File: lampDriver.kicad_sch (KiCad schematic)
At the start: 49 parts, among them IC8 FAN3100TSX, T4 NMOS_GDS-KS_SMD, U1 OPA2356AIDGKR, U3 LM2903, U4 AZ431LANTR

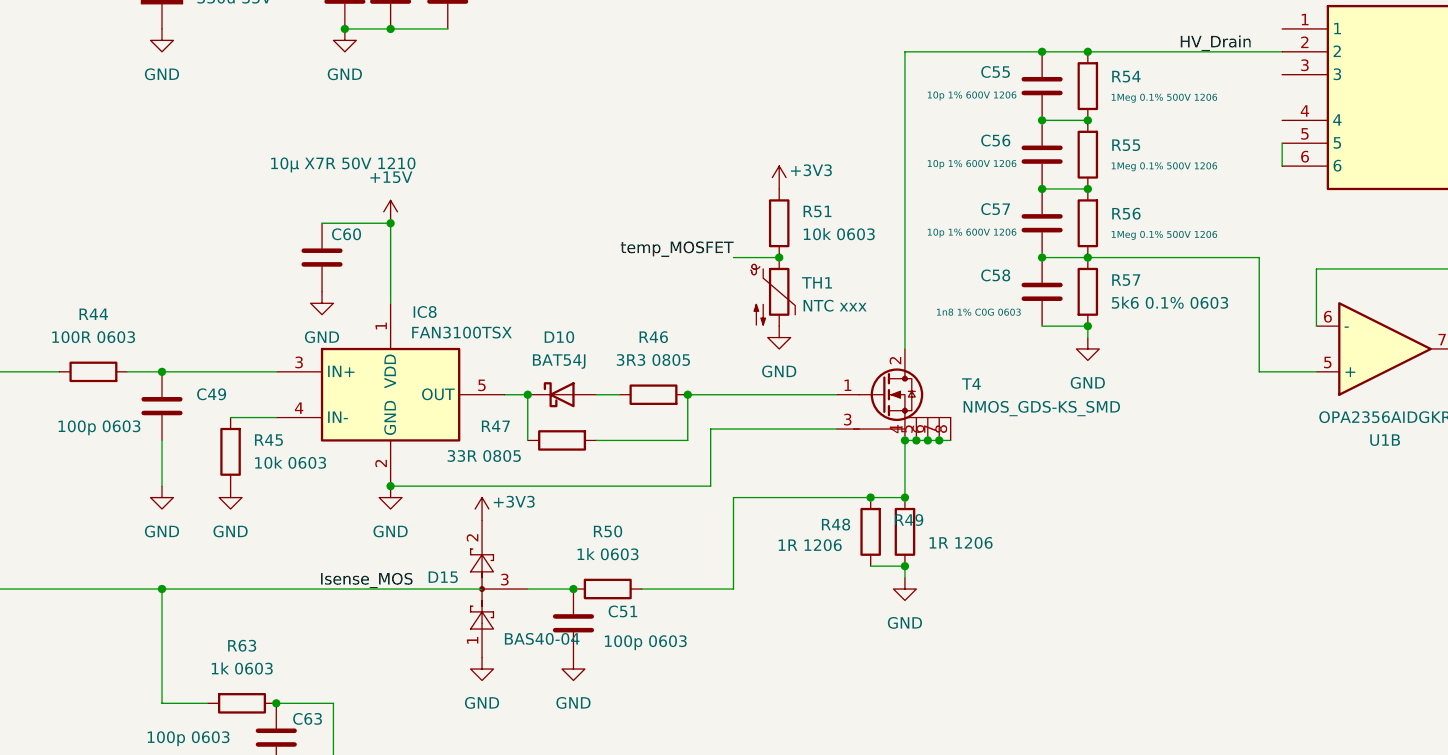
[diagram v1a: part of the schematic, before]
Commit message: 250415_endOfDay
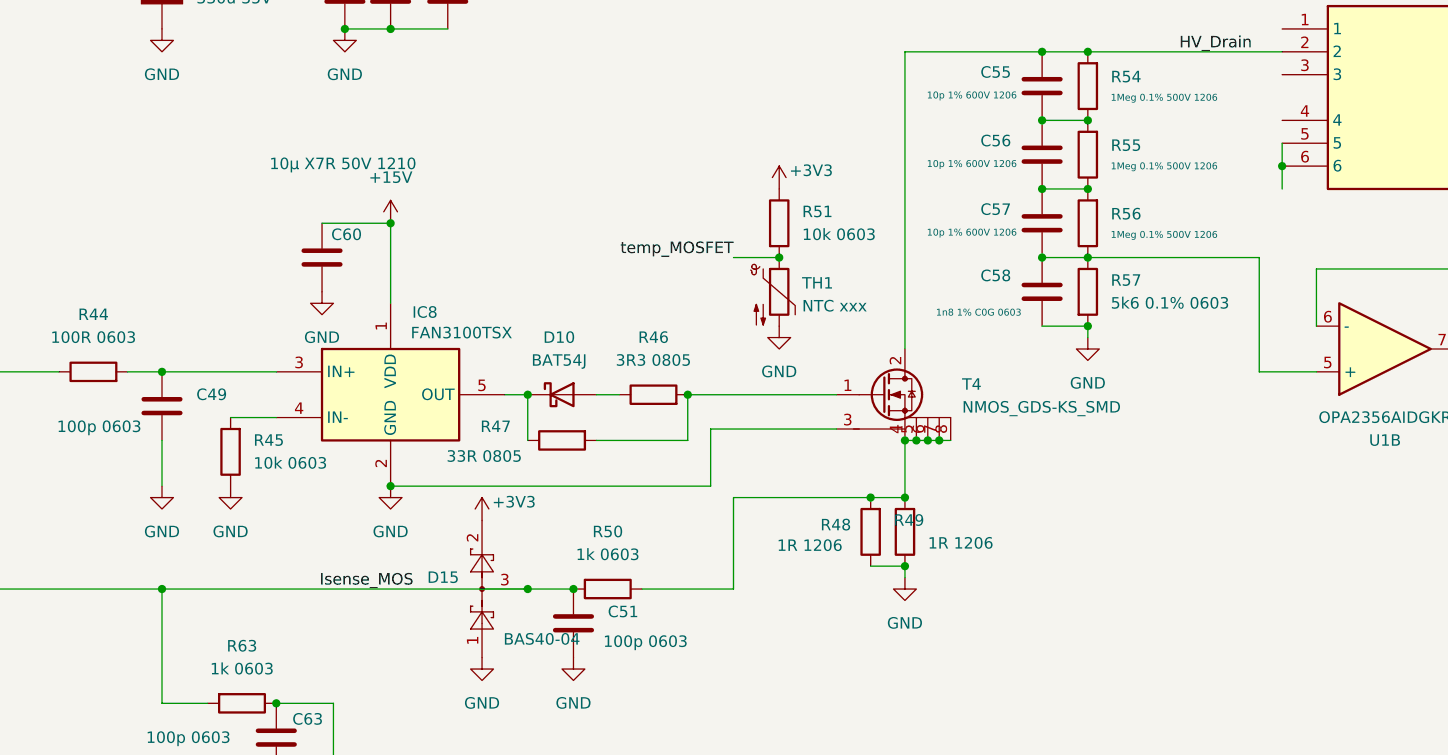
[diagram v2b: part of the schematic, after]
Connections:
- net Isense_MOS: now also C51.1, D15.3, R50.2
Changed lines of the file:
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@@
+	)
+	(junction
+		(at 175.26 60.96)
+		(diameter 0)
+		(color 0 0 0 0)
 	)
 	(junction
@@
 	)
 	(junction
+		(at 91.44 107.95)
+		(diameter 0)
+		(color 0 0 0 0)
+	)
+	(junction
 		(at 76.2 67.31)
 		(diameter 0)
@@
 	(wire
 		(pts
+			(xy 175.26 60.96) (xy 175.26 63.5)
+		)
+		(stroke
+			(width 0)
+			(type default)
+		)
+	)
+	(wire
+		(pts
 			(xy 208.28 50.8) (xy 208.28 71.12)
 		)
@@
 	(wire
 		(pts
-			(xy 50.8 107.95) (xy 86.36 107.95)
+			(xy 50.8 107.95) (xy 91.44 107.95)
 		)
 		(stroke
@@
 			(fill
 				(type none)
+			)
+		)
+	)
+	(netclass_flag ""
+		(length 2.54)
+		(shape round)
+		(at 153.67 63.5 270)
+		(effects
+			(font
+				(size 1.27 1.27)
+			)
+			(justify right bottom)
+		)
+		(property "Net Class" "HV_Drain_div2"
+			(at 157.734 63.246 0)
+			(effects
+				(font
+					(size 1.27 1.27)
+				)
+				(justify left)
+			)
+		)
+		(property "Component Class" ""
+			(at -49.53 8.89 0)
+			(effects
+				(font
+					(size 1.27 1.27)
+					(italic yes)
+				)
+			)
+		)
+	)
+	(netclass_flag ""
+		(length 2.54)
+		(shape round)
+		(at 153.67 55.88 270)
+		(effects
+			(font
+				(size 1.27 1.27)
+			)
+			(justify right bottom)
+		)
+		(property "Net Class" "HV_Drain_div"
+			(at 157.226 55.88 0)
+			(effects
+				(font
+					(size 1.27 1.27)
+				)
+				(justify left)
+			)
+		)
+		(property "Component Class" ""
+			(at -48.26 1.27 0)
+			(effects
+				(font
+					(size 1.27 1.27)
+					(italic yes)
+				)
+			)
+		)
+	)
+	(netclass_flag ""
+		(length 2.54)
+		(shape round)
+		(at 175.26 63.5 180)
+		(fields_autoplaced yes)
+		(effects
+			(font
+				(size 1.27 1.27)
+			)
+			(justify right bottom)
+		)
+		(property "Net Class" "HV_Lamp/2"
+			(at 175.9585 66.04 0)
+			(effects
+				(font
+					(size 1.27 1.27)
+				)
+				(justify left)
+			)
+		)
+		(property "Component Class" ""
+			(at -44.45 31.75 0)
+			(effects
+				(font
+					(size 1.27 1.27)
+					(italic yes)
+				)
 			)
 		)
@@
 			(effects
 				(font
+					(size 1.27 1.27)
+					(italic yes)
+				)
+			)
+		)
+	)
+	(netclass_flag ""
+		(length 2.54)
+		(shape round)
+		(at 214.63 22.86 0)
+		(fields_autoplaced yes)
+		(effects
+			(font
+				(size 1.27 1.27)
+			)
+			(justify left bottom)
+		)
+		(property "Net Class" "HV_Lamp"
+			(at 215.3285 20.32 0)
+			(effects
+				(font
+					(size 1.27 1.27)
+				)
+				(justify left)
+			)
+		)
+		(property "Component Class" ""
+			(at -73.66 -6.35 0)
+			(effects
+				(font
